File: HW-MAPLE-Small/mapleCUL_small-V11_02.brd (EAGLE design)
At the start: 80 x 30 mm, 18 parts, among them IC2 LAN-USR-ES1

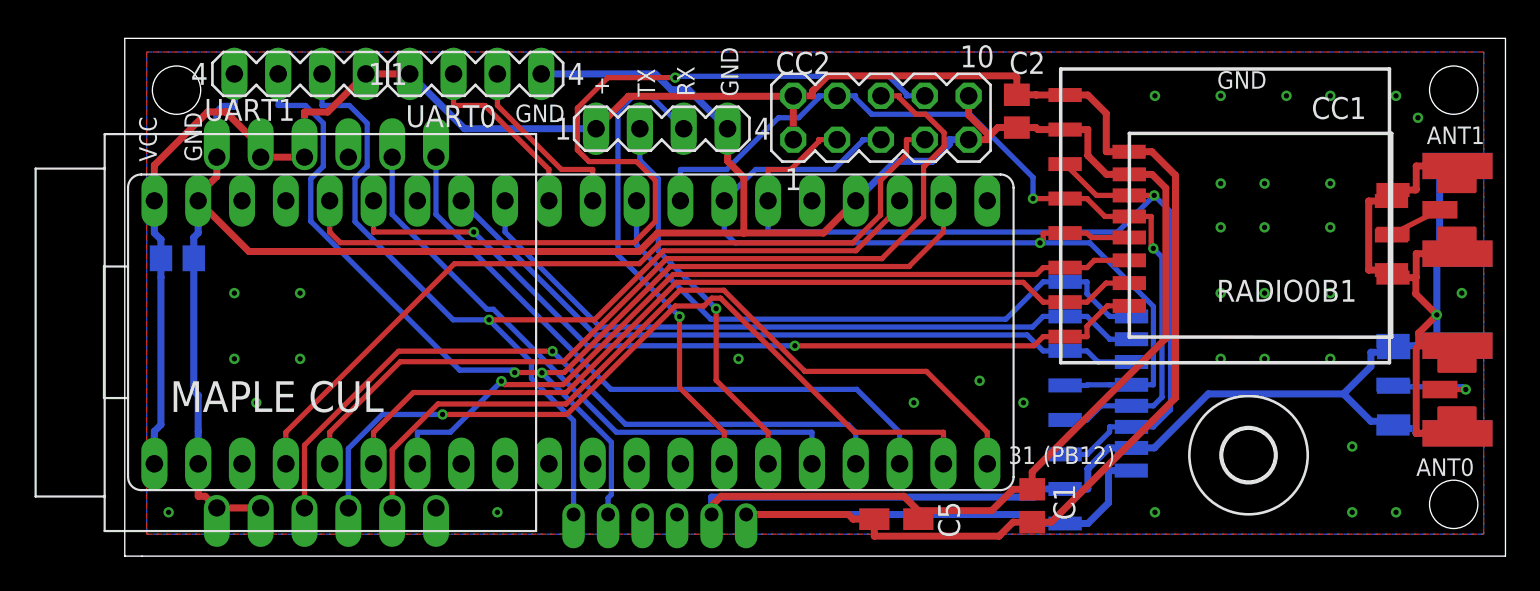
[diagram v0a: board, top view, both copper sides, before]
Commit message: Small + Zigbee
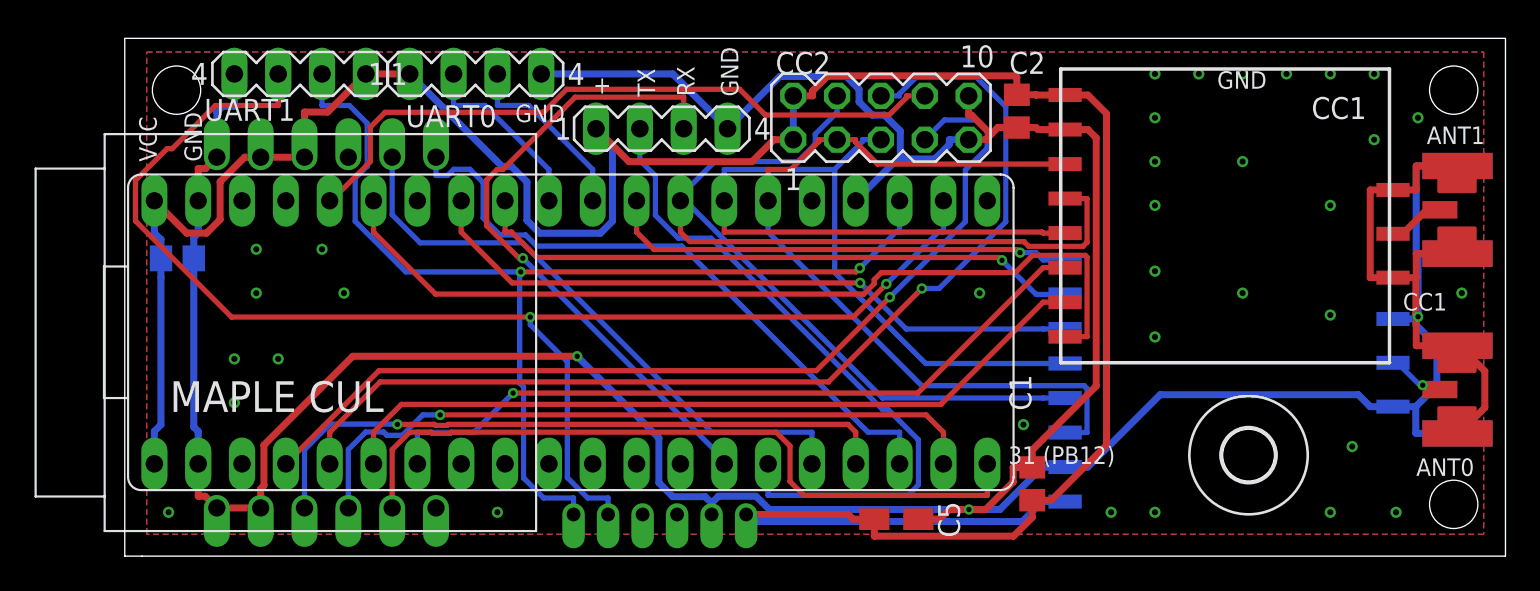
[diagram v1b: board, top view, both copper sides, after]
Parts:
- removed RADIO0B: CC1101_MODULE1SMALL, Martin-Communication:CC1101_MODULE1_SMD
- removed RADIO0B1: CC1101_MODULE1SMD, Martin-Communication:CC1101_MODULE1_SMD
- moved CC0 1.27 mm to (54.5, 17.2)
- moved C1 1.27 mm to (52.6, 4.19)
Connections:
- net ANT1: no longer RADIO0B1.ANT
- net ANT2: no longer RADIO0B.ANT
- net CC_CS0: no longer RADIO0B.CSN
- net CC_CS1: no longer RADIO0B1.CSN
- net CC_IN_0: no longer RADIO0B.GDO2
- net CC_IN_1: no longer RADIO0B1.GDO2
- net CC_OUT_0: no longer RADIO0B.GDO0
- net CC_OUT_1: no longer RADIO0B1.GDO0
- net GND: no longer RADIO0B.GND@0, RADIO0B.GND@1, RADIO0B.GND@2, RADIO0B1.GND@0, RADIO0B1.GND@1, RADIO0B1.GND@2
- net MISO1: no longer RADIO0B.MISO, RADIO0B1.MISO
- net MOSI1: no longer RADIO0B.MOSI, RADIO0B1.MOSI
- net SCK1: no longer RADIO0B.SCLK, RADIO0B1.SCLK
- net VCC: no longer RADIO0B.VCC, RADIO0B1.VCC
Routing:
- net SCK1: track 51.5 -> 69.5 mm, vias 2 -> 0
- net TX_DBG: track 22.5 -> 39.4 mm, vias 1 -> 0
- net RX1: track 66.3 -> 81.2 mm
- net GND: track 258.4 -> 243.8 mm, vias 35 -> 37
- net CC_OUT_2: track 52.9 -> 39.5 mm, vias 1 -> 0
- net CC_IN_2: track 51.4 -> 61.2 mm, vias 0 -> 1
- net RX_DBG: track 27.9 -> 37.5 mm
- net MOSI1: track 57.7 -> 48.3 mm, vias 1 -> 0
- net CC_CS0: track 35.1 -> 27.3 mm, vias 0 -> 1
- net CC_CS2: track 47.5 -> 55.3 mm, vias 0 -> 1
- net SCK2: track 46.6 -> 41.1 mm
- net CC_OUT_0: track 41.2 -> 35.8 mm, vias 0 -> 1
- net CC_OUT_1: track 50.1 -> 45.0 mm
- net CC_IN_1: track 47.4 -> 43.3 mm
- net WIZ_CS: track 46.9 -> 42.9 mm
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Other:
- board text added: "CC0"
- board text added: "CC1"
- board text added: "Small V1.1 www.neuby.de"
- board text removed: "Small V1.0 www.neuby.de"
